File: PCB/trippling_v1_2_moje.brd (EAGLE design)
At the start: 55.9 x 26.7 mm, 24 parts, among them K3 2071508-1, K4 2071508-1, T1 MMBT3904, T2 MMBT3904, X1 1751277

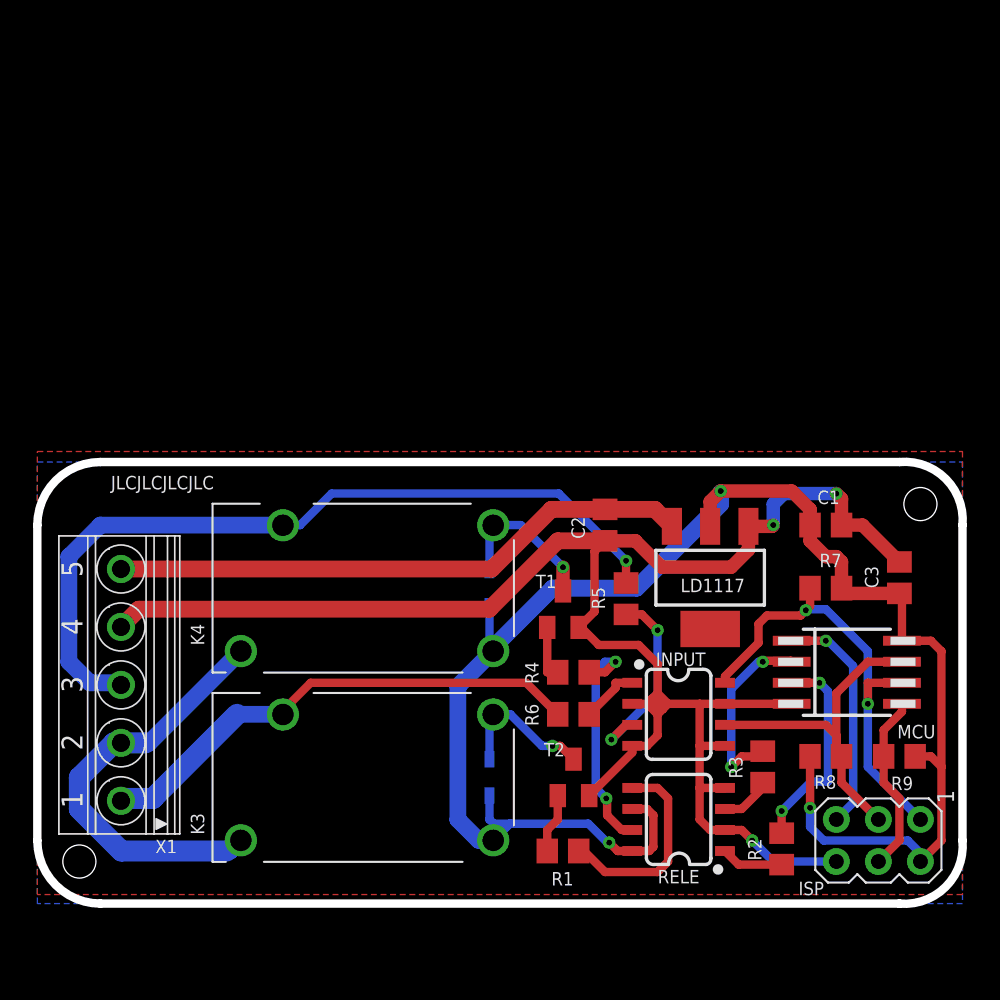
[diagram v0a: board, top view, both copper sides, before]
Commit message: As built
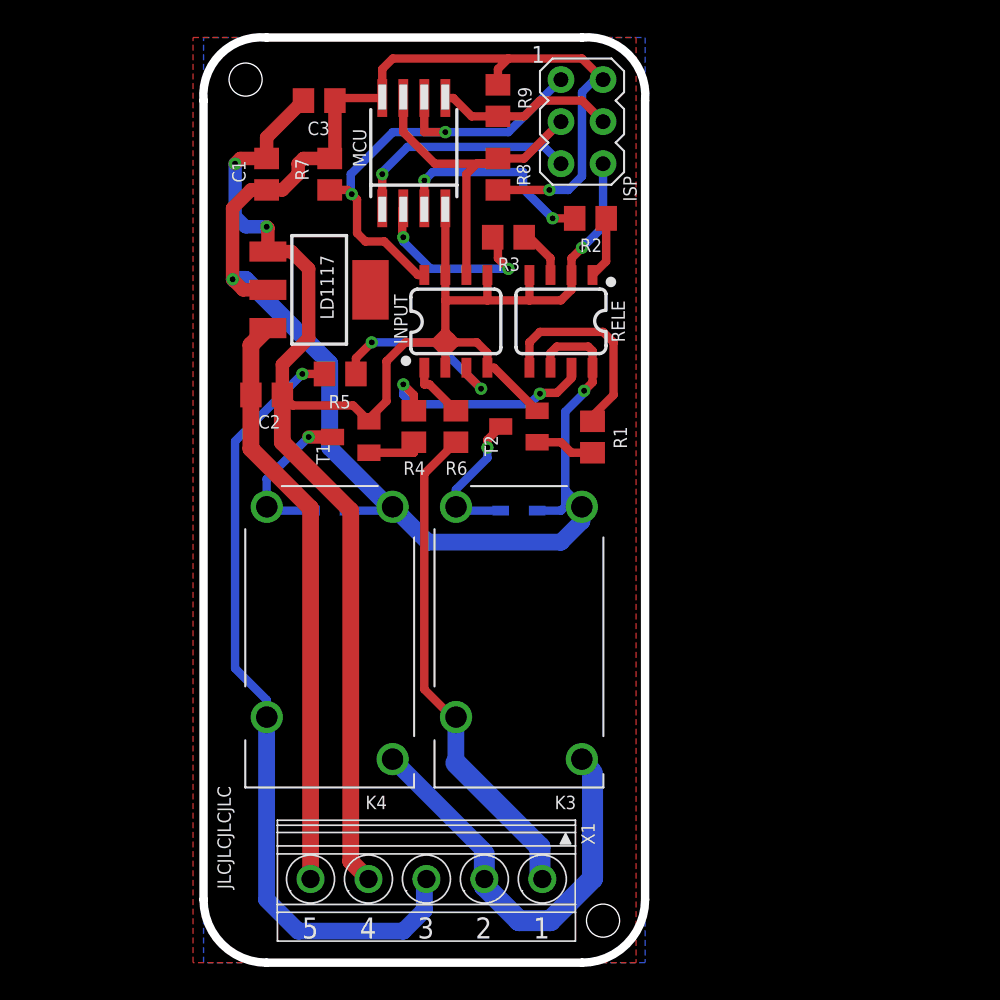
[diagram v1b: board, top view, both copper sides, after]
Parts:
- moved ISP 47.0 mm to (35.4, 122.2), turned to 0 degrees
- moved R9 46.4 mm to (30.4, 123.4), turned to 90 degrees
- moved C3 45.4 mm to (19.6, 123.4), turned to 180 degrees
- moved MCU 40.8 mm to (25.3, 120.3), turned to 0 degrees
- moved R8 40.4 mm to (30.4, 119.0), turned to 270 degrees
- moved C1 39.9 mm to (16.4, 119.0), turned to 90 degrees
- moved R2 39.8 mm to (35.9, 116.3), turned to 0 degrees
- moved R7 39.0 mm to (20.2, 119.0), turned to 90 degrees
- moved R3 35.5 mm to (31.0, 115.2), turned to 0 degrees
- moved RELE 30.9 mm to (34.2, 110.1), turned to 180 degrees
- moved LD1117 29.3 mm to (19.6, 112.0), turned to 270 degrees
- moved INPUT 27.3 mm to (27.8, 110.1), turned to 0 degrees
- moved R1 25.1 mm to (36.1, 103.1), turned to 270 degrees
- moved X1 22.0 mm to (26.0, 76.3), turned to 180 degrees
- moved R5 22.0 mm to (20.8, 106.9), turned to 180 degrees
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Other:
- board size 55.9 x 26.7 mm -> 26.7 x 55.9 mm
